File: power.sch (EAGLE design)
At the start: 32 parts, among them IC1 74HC125D, IC2 7805TV, IC3 7815TV

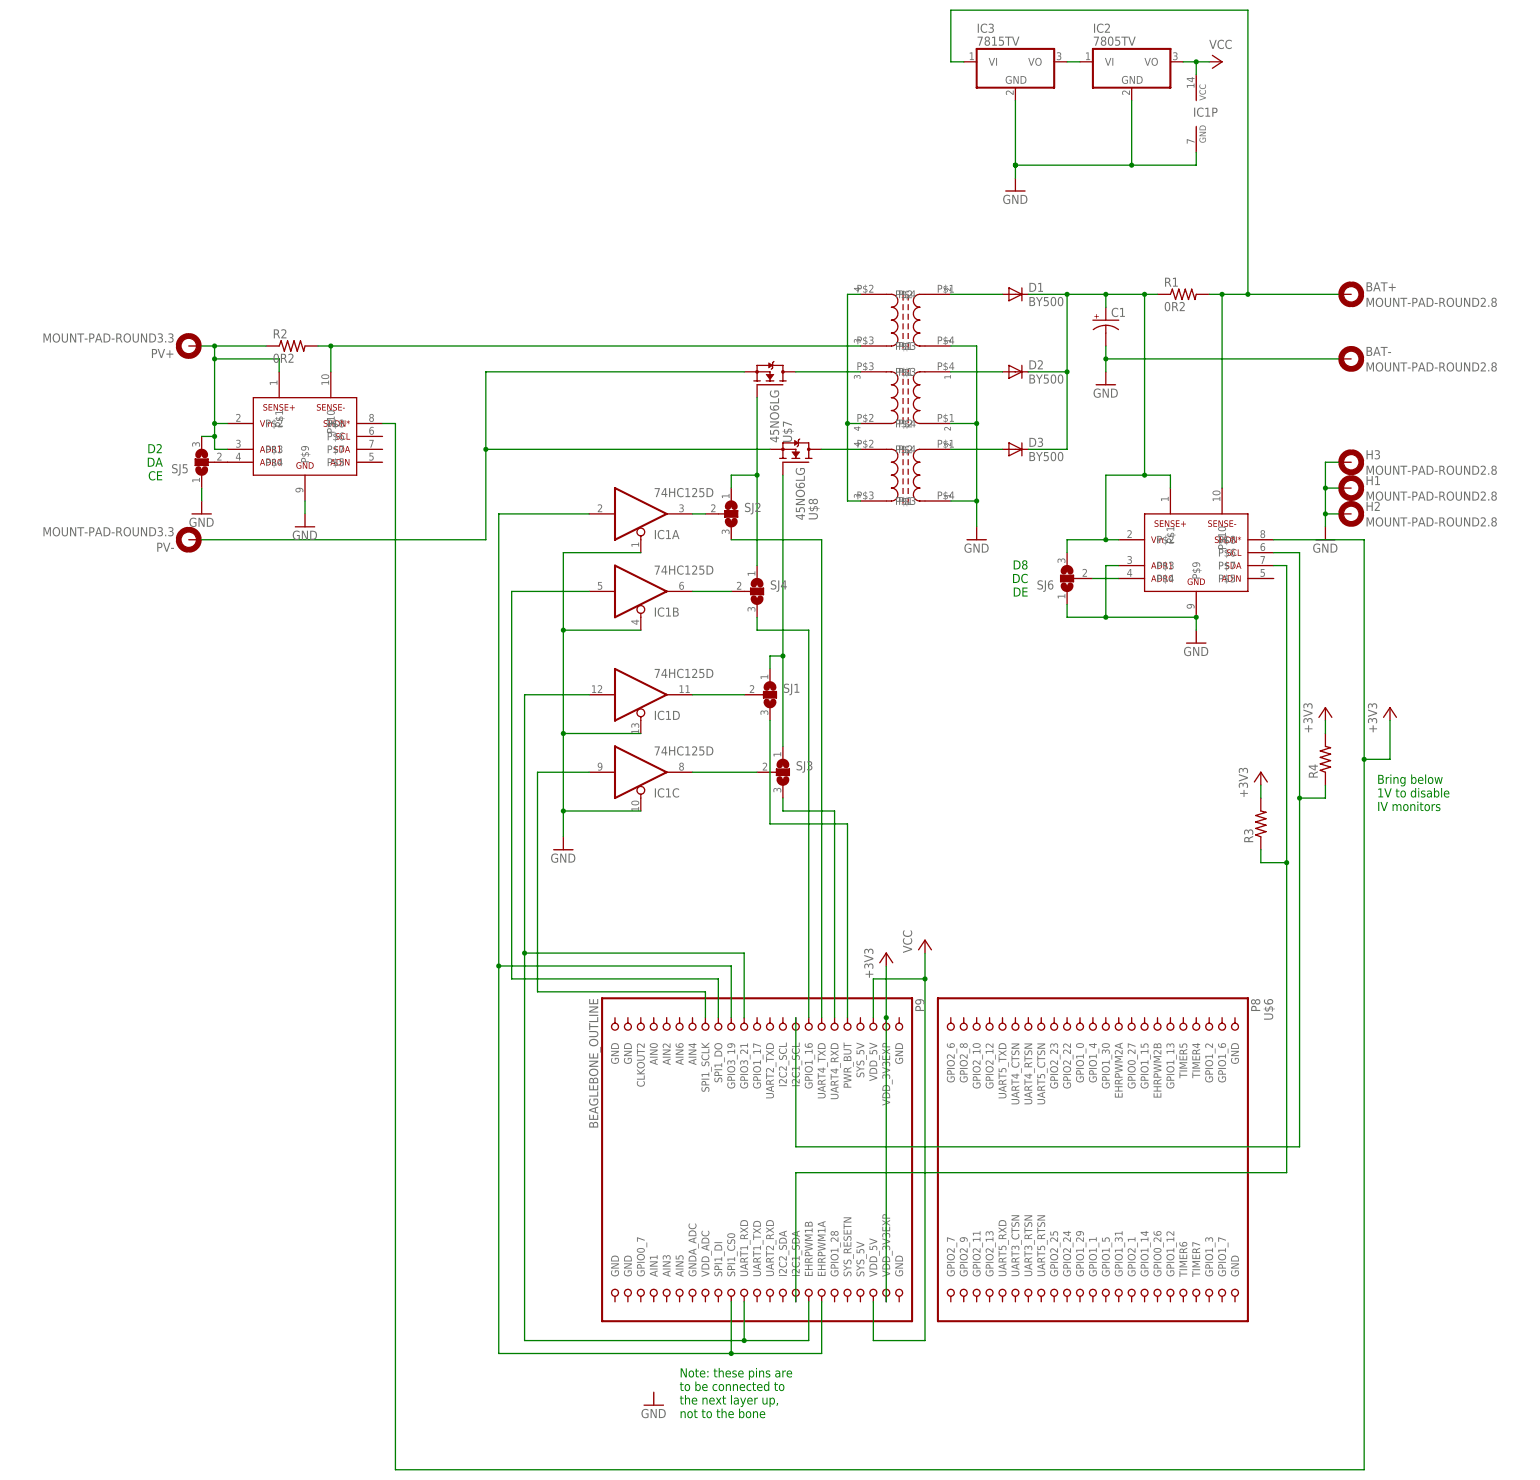
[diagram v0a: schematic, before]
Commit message: whomp
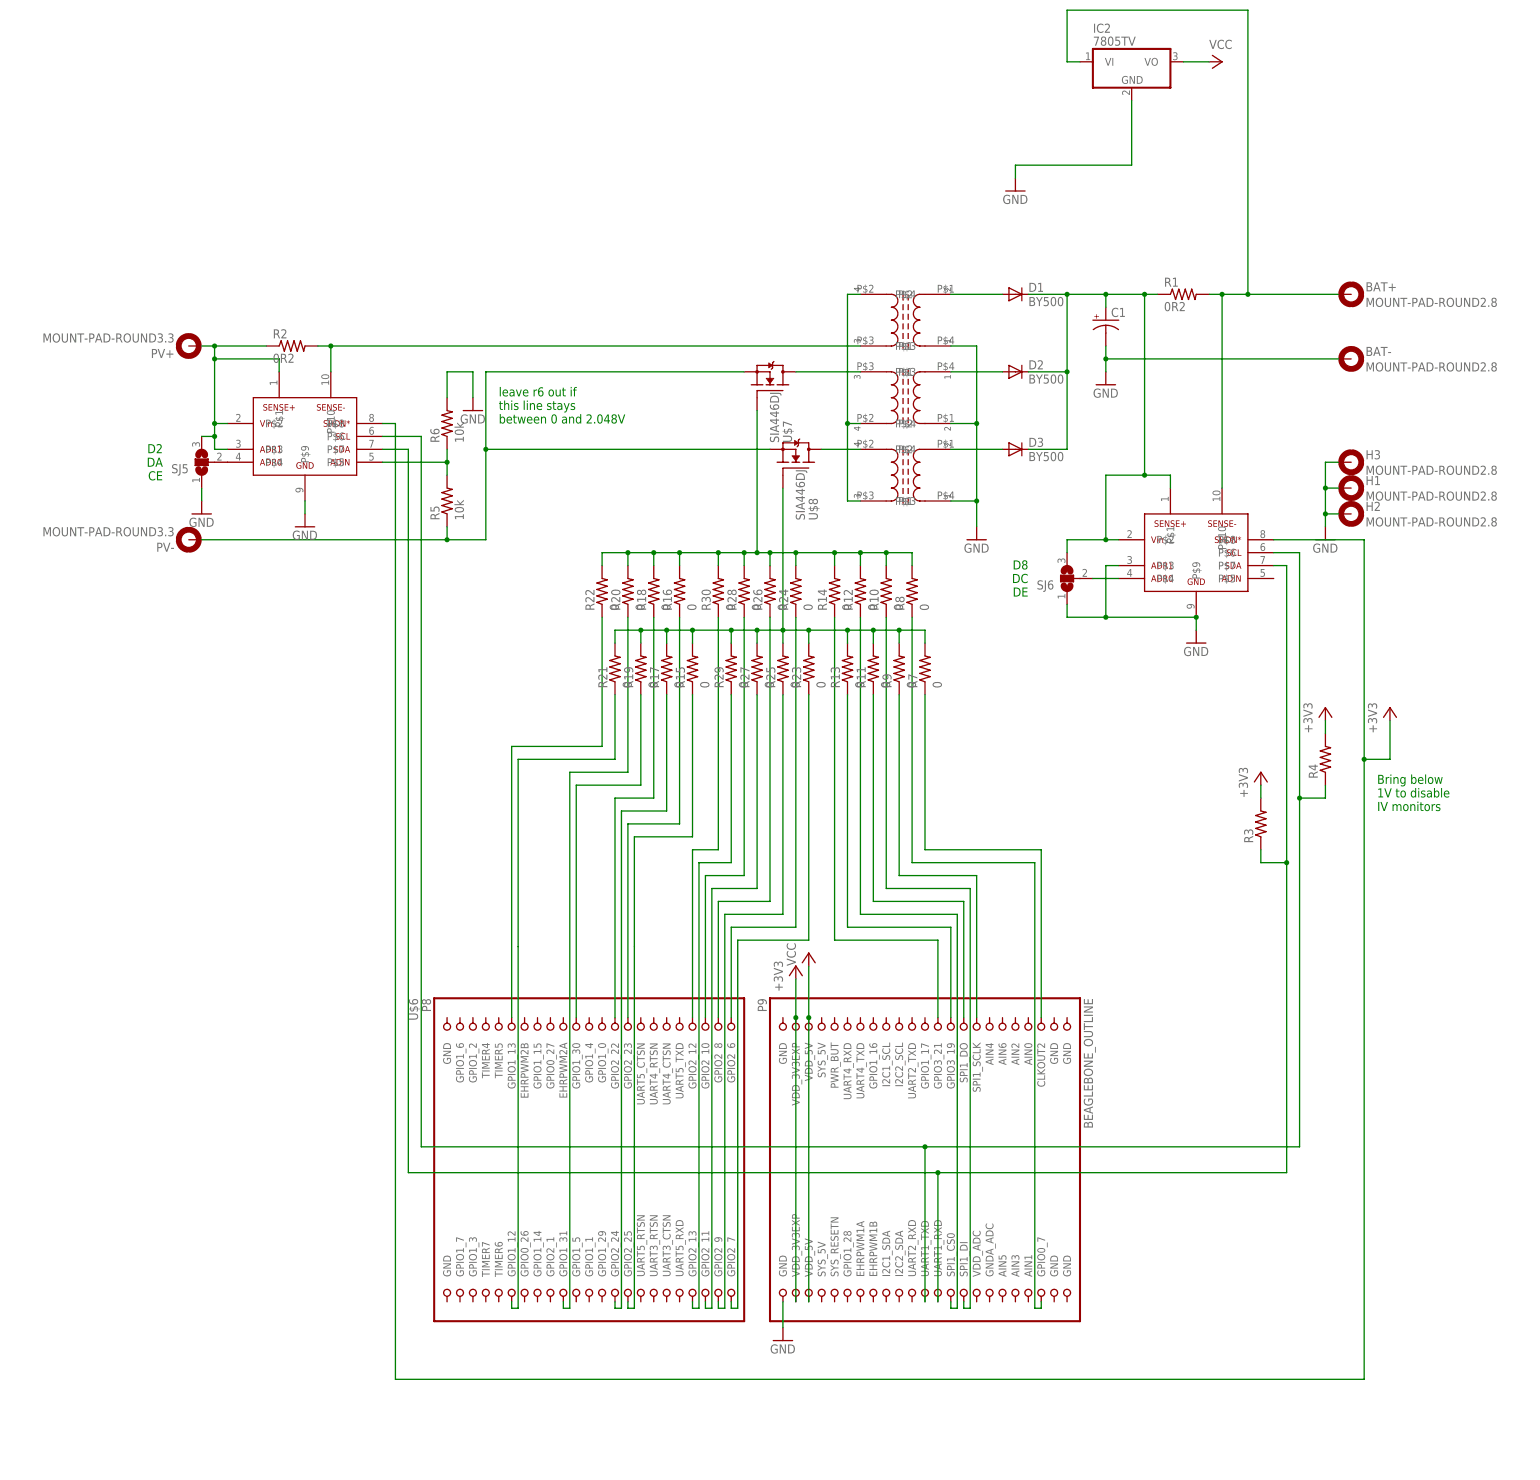
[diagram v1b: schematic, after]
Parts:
- removed IC1: 74HC125D, 74xx-eu:74HC125D
- removed IC3: 7815TV, linear:7815TV
- removed SJ1, SJ2, SJ3, SJ4: (no value), jumper:SJ2W
- added R10, R11, R12, R13, R14, R15, R16, R17, R18, R19, R20, R21, R22, R23, R24, R25, R26, R27, R28, R29, R30, R7, R8, R9: 0, rcl:R-US_R0603
- added R5, R6: 10k, rcl:R-US_R0603
- U$7, U$8: value 45NO6LG -> SIA446DJ; device semiconductors:45NO6LG -> semiconductors:SIA446DJ
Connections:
- removed net N$27: IC2.VI, IC3.VO
- new net N$17: R9.1, U$6.SPI1_SCLK
- new net N$18: R10.1, U$6.SPI1_DI
- new net N$30: R5.2, R6.1, U$1.P$5
- new net N$31: R26.1, U$6.GPIO2_8
- new net N$32: R27.1, U$6.GPIO2_11
- new net N$34: R29.1, U$6.GPIO2_13
- new net N$35: R30.1, U$6.GPIO2_12
- new net N$36: U$6.GPIO1_12
- new net N$39: R19.1, U$6.GPIO1_30
- new net N$40: R18.1, U$6.GPIO2_22
- new net N$41: R17.1, U$6.GPIO2_24
- new net N$42: R16.1, U$6.GPIO2_23
- new net N$43: U$6.GPIO2_25
- new net N$44: R10.2, R12.2, R14.2, R16.2, R18.2, R20.2, R22.2, R24.2, R26.2, R28.2, R30.2, R8.2, U$7.G
- new net N$45: R11.2, R13.2, R15.2, R17.2, R19.2, R21.2, R23.2, R25.2, R27.2, R29.2, R7.2, R9.2, U$8.G
- net GND: now also R6.2, U$6.GND@2; no longer IC1A.OE, IC1B.OE, IC1C.OE, IC1D.OE, IC1P.GND, IC3.GND
- net N$11: now also R15.1; no longer SJ1.1, SJ3.1, U$8.G
- net N$13: now also R21.1; no longer SJ2.1, SJ4.1, U$7.G
- net N$14: now also U$1.P$6, U$6.UART1_TXD; no longer U$6.I2C1_SCL
- net N$19: now also R11.1, U$6.SPI1_DO; no longer SJ1.3, U$6.PWR_BUT
- net N$20: now also R7.1, U$6.CLKOUT2; no longer IC1A.O, SJ2.2
- net N$21: now also R8.1, U$6.GPIO0_7; no longer SJ3.3, U$6.UART4_RXD
- net N$22: now also R12.1, U$6.SPI1_CS0; no longer SJ4.3, U$6.GPIO1_16
- net N$23: now also R13.1; no longer IC1A.I, U$6.EHRPWM1A, U$6.SPI1_CS0
- net N$24: now also R14.1, U$6.GPIO3_21; no longer IC1B.O, SJ4.2
- net N$25: now also R23.1, U$6.GPIO2_7; no longer IC1D.O, SJ1.2
- net N$28: now also R24.1, U$6.GPIO2_6; no longer IC1D.I, U$6.EHRPWM1B, U$6.GPIO3_21, U$6.UART1_RXD
- net N$29: now also R25.1, U$6.GPIO2_9; no longer IC1C.O, SJ3.2
- net N$33: now also R28.1, U$6.GPIO2_10; no longer SJ2.3, U$6.UART4_TXD
- net N$37: now also R22.1, U$6.GPIO1_13; no longer IC1B.I, U$6.SPI1_DO
- net N$38: now also R20.1, U$6.GPIO1_31; no longer IC1C.I, U$6.SPI1_SCLK
- net N$4: now also IC2.VI; no longer IC3.VI
- net N$7: now also U$1.P$7, U$6.UART1_RXD; no longer U$6.I2C1_SDA
- net N$8: now also R5.1
- net VCC: no longer IC1P.VCC
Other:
- note added: "leave r6 out if this line stays between 0 and 2.048V"
- note removed: "Note: these pins are to be connected to the next layer up, not to the bone"
- moved on the sheet: U$6
